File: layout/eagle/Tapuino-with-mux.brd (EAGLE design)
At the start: 100 x 80 mm, 13 parts, among them CN1 C64_CASETTE_EDGE, IC1 4052N

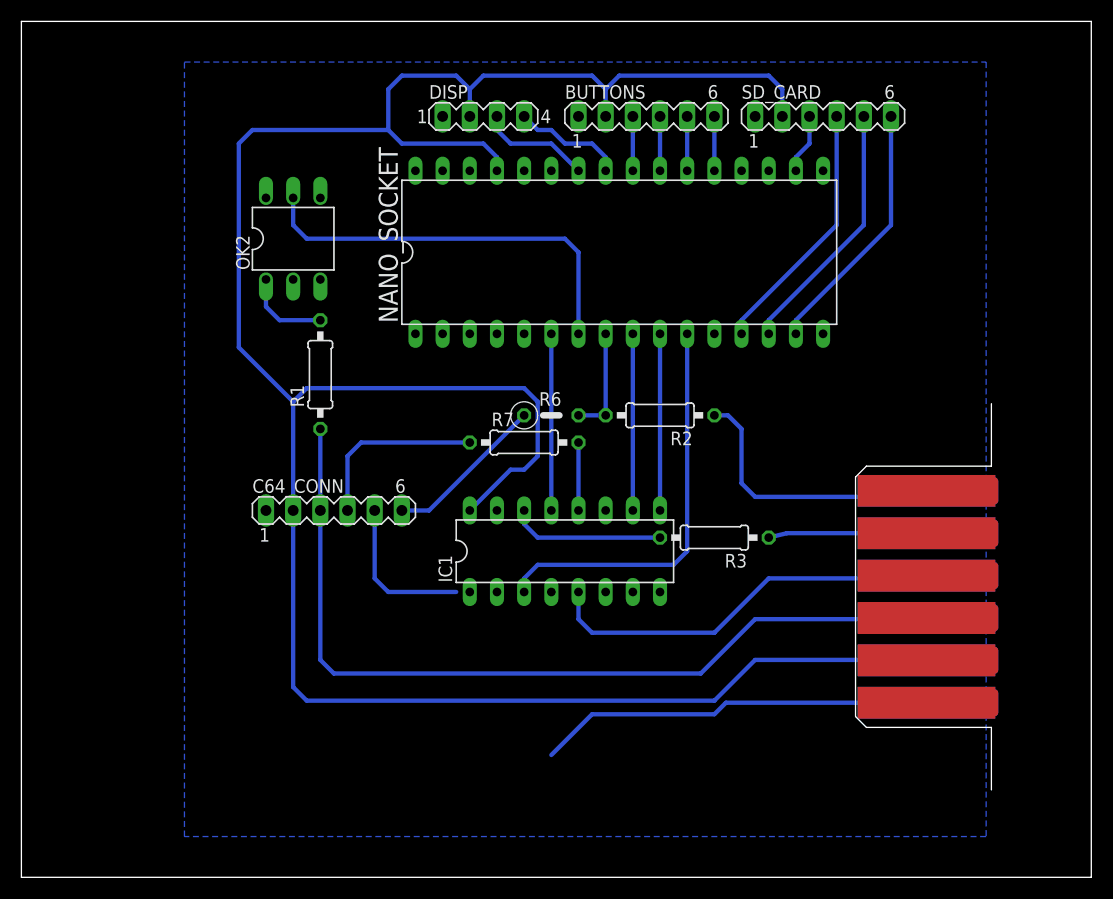
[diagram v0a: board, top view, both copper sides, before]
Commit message: Minor changes to mux board
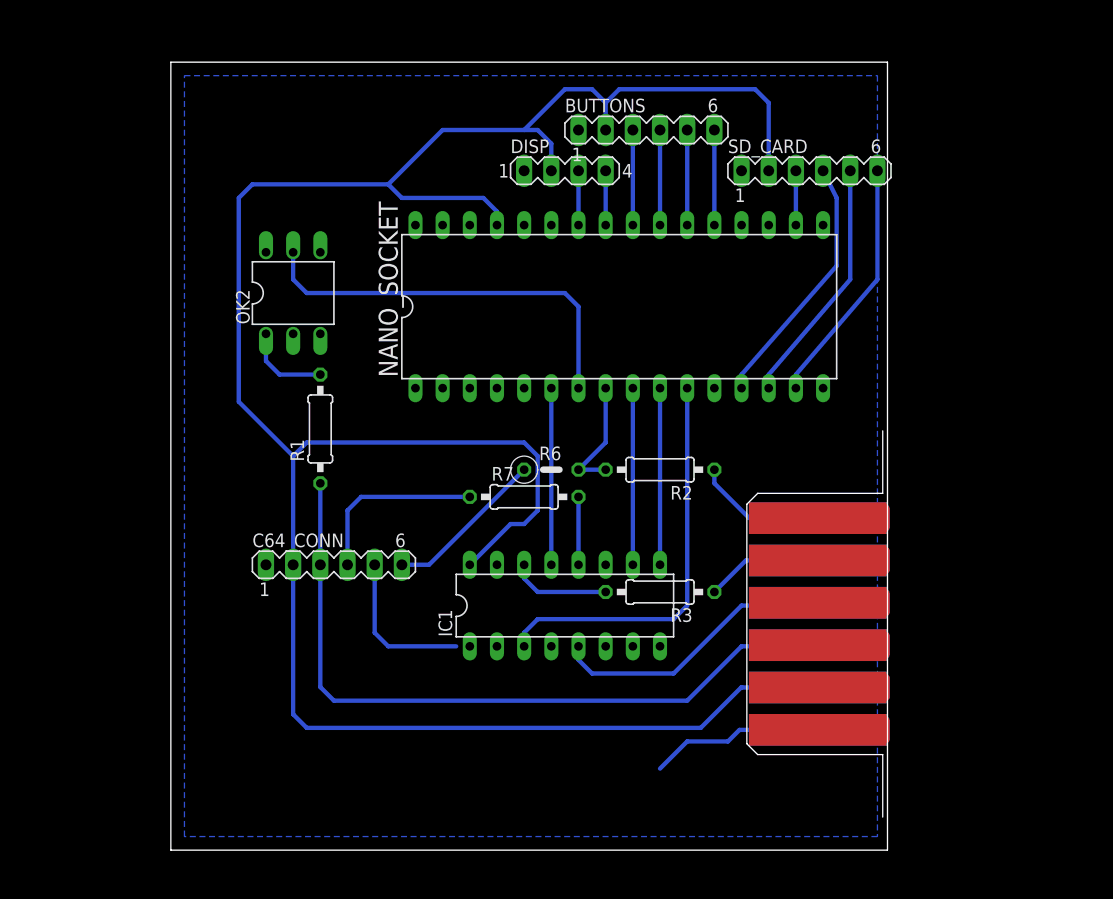
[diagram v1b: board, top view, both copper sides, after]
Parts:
- moved CN1 10.5 mm to (74.9, 35.6)
- moved DISP 9.16 mm to (50.8, 66.0)
- moved R3 7.18 mm to (59.7, 26.7)
- moved SD_CARD 5.24 mm to (73.7, 66.0)
- moved R1 5.08 mm to (27.9, 41.9)
- moved IC1 5.08 mm to (50.8, 25.4)
- moved C64_CONN 5.08 mm to (29.2, 29.2)
- moved NANO_SOCKET 5.08 mm to (55.9, 53.3)
- moved OK2 5.08 mm to (25.4, 54.6)
- moved R2 5.08 mm to (59.7, 38.1)
- moved R6 5.08 mm to (49.5, 38.1)
- moved R7 5.08 mm to (47.0, 35.6)
- moved BUTTONS 1.27 mm to (58.4, 69.8)
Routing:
- net GND: track 41.3 -> 20.4 mm
- net D5/S_0OHM2: track 30.5 -> 16.5 mm
- net DAT/READ: track 41.9 -> 31.1 mm
- net MOTOR: track 85.1 -> 75.2 mm
- net VCC: track 234.2 -> 225.4 mm
- net A5/SCL: track 10.5 -> 5.08 mm
- net A4/SDA: track 10.5 -> 5.08 mm
- net DAT/WRITE: track 14.5 -> 9.42 mm
- net D/W_0OHM: track 19.0 -> 15.1 mm
- net A3/BTN1: track 5.08 -> 8.89 mm
- net A2/BTN2: track 5.08 -> 8.89 mm
- net A1/BTN3: track 5.08 -> 8.89 mm
- net A0/BTN4: track 5.08 -> 8.89 mm
- net D5/SENSE: track 10.2 -> 11.2 mm
- net D12/MISO: track 24.0 -> 23.1 mm
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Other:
- board size 100 x 80 mm -> 67 x 73.6 mm
